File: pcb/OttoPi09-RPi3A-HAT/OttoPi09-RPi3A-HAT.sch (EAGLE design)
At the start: 46 parts, among them Q1 2SK4017

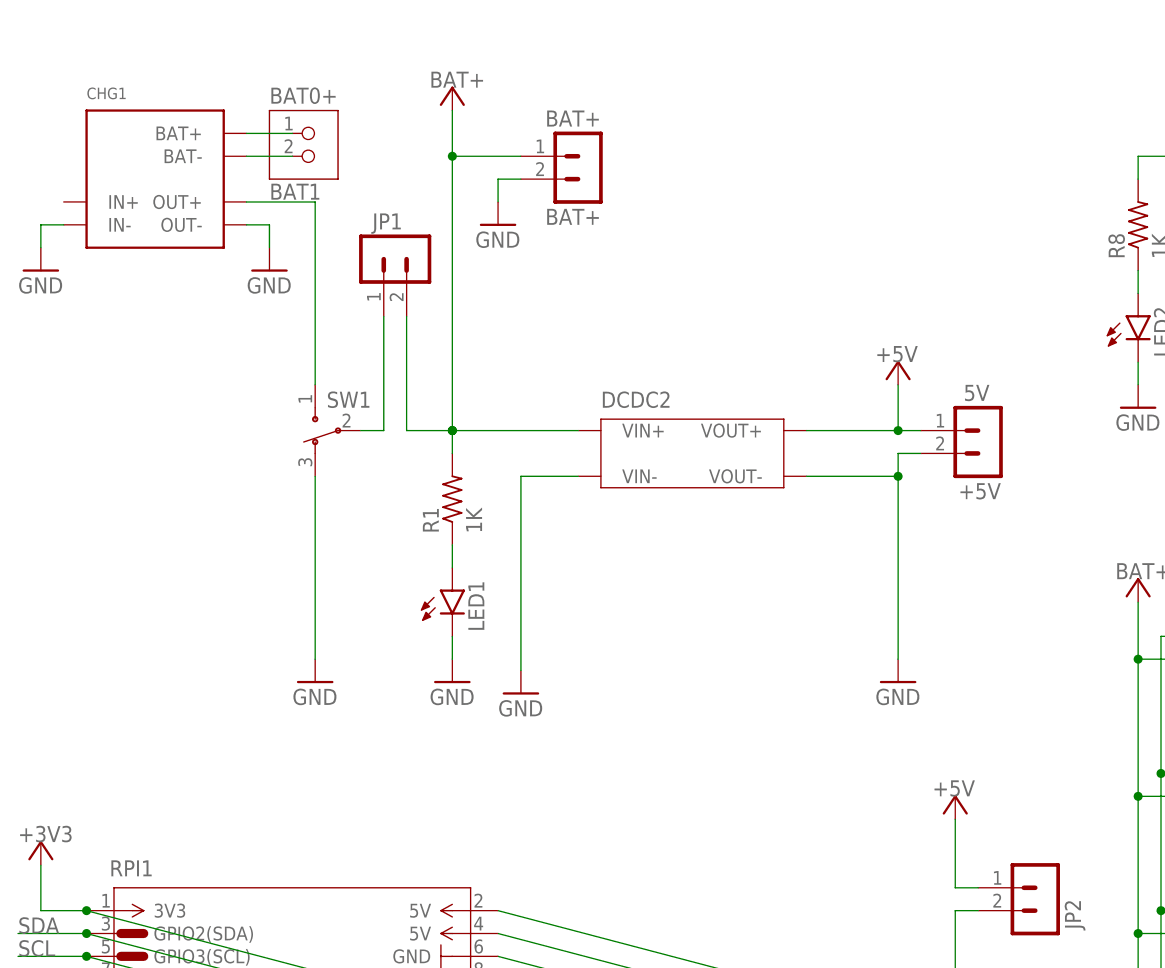
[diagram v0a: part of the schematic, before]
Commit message: UPD: pcb
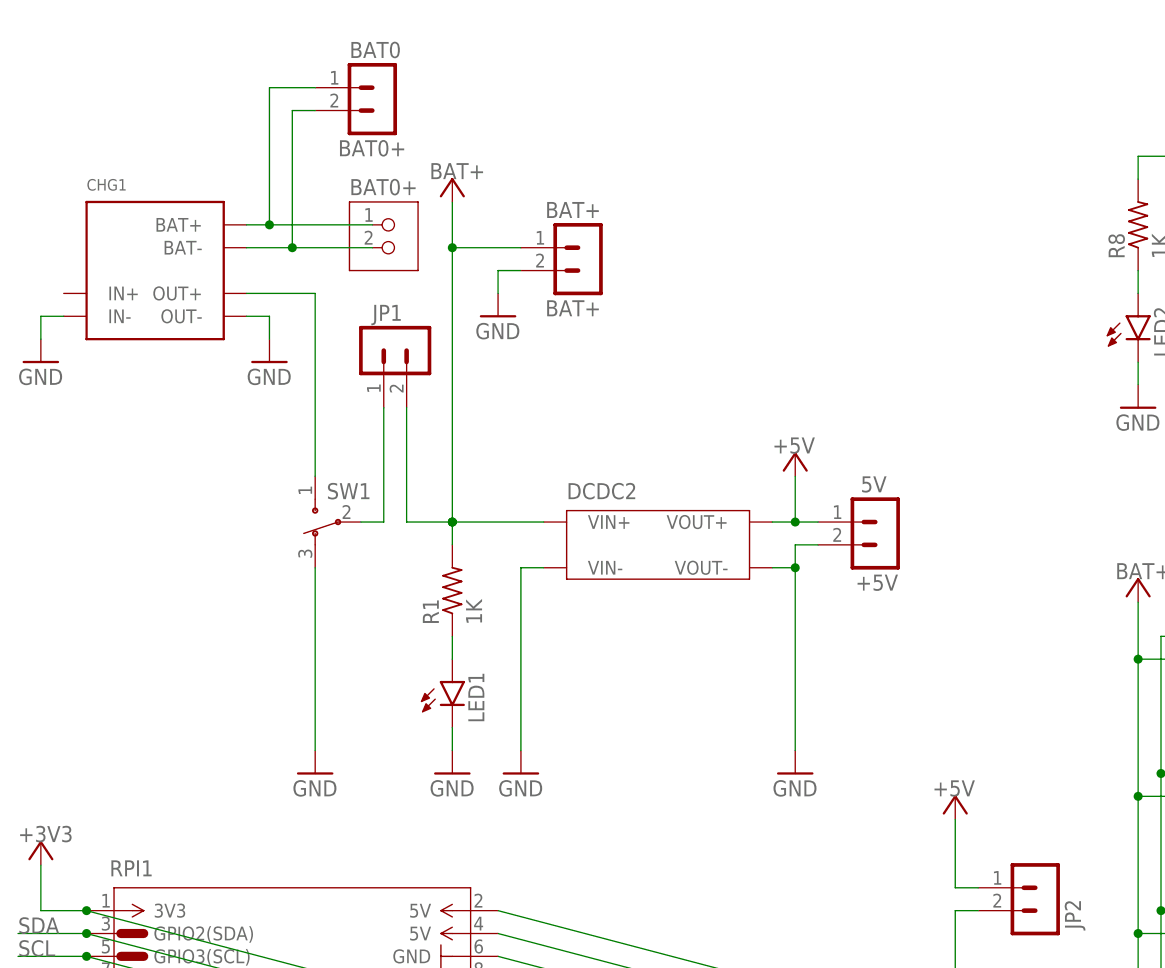
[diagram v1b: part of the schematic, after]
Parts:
- added BAT0: BAT0+, ytani1:PINHEAD-MA02-1
- BAT0+: value BAT1 -> (none)
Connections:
- net BAT+0: now also BAT0.1
- net BAT-0: now also BAT0.2
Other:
- moved on the sheet: +5V, BAT+, BAT0+, CHG1, DCDC2, JP1, LED1, R1, SW1
